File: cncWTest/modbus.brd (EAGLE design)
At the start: 39.4 x 34 mm, 12 parts, among them Q2 2N3904

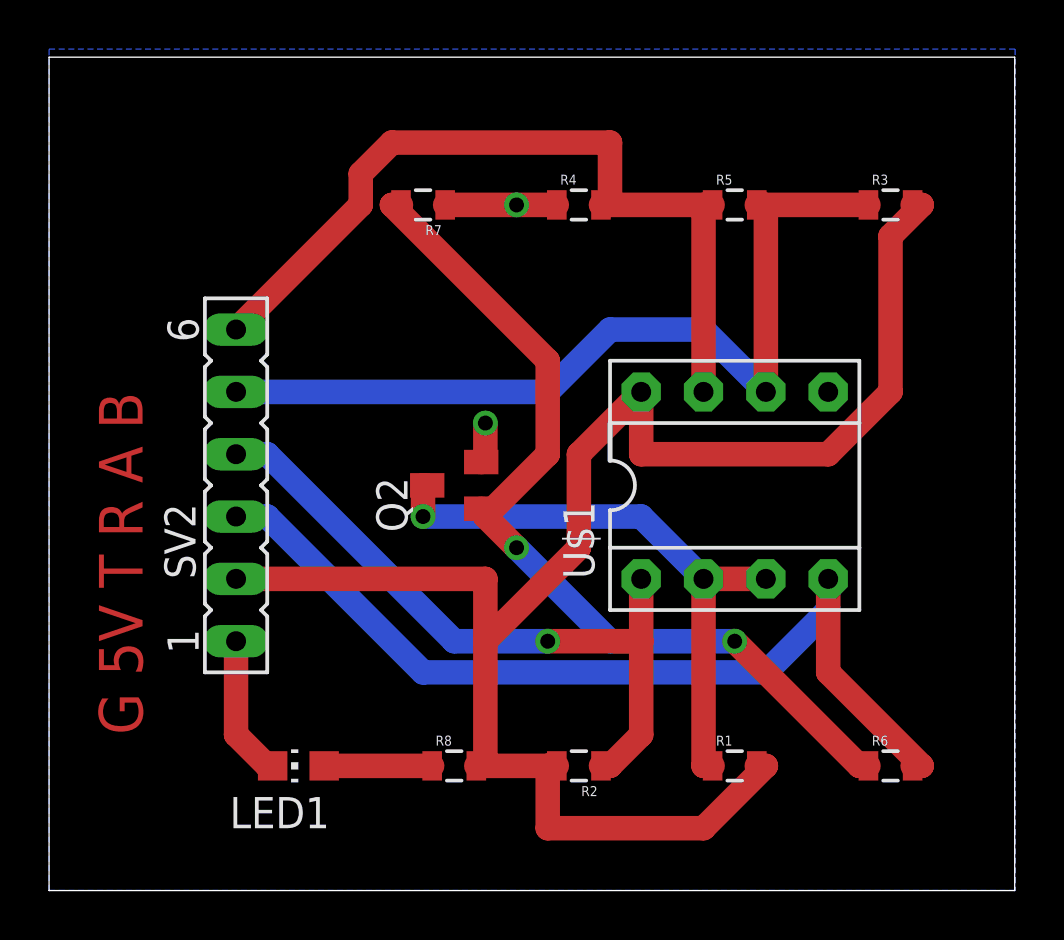
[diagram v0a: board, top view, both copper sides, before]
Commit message: CNC conf 1
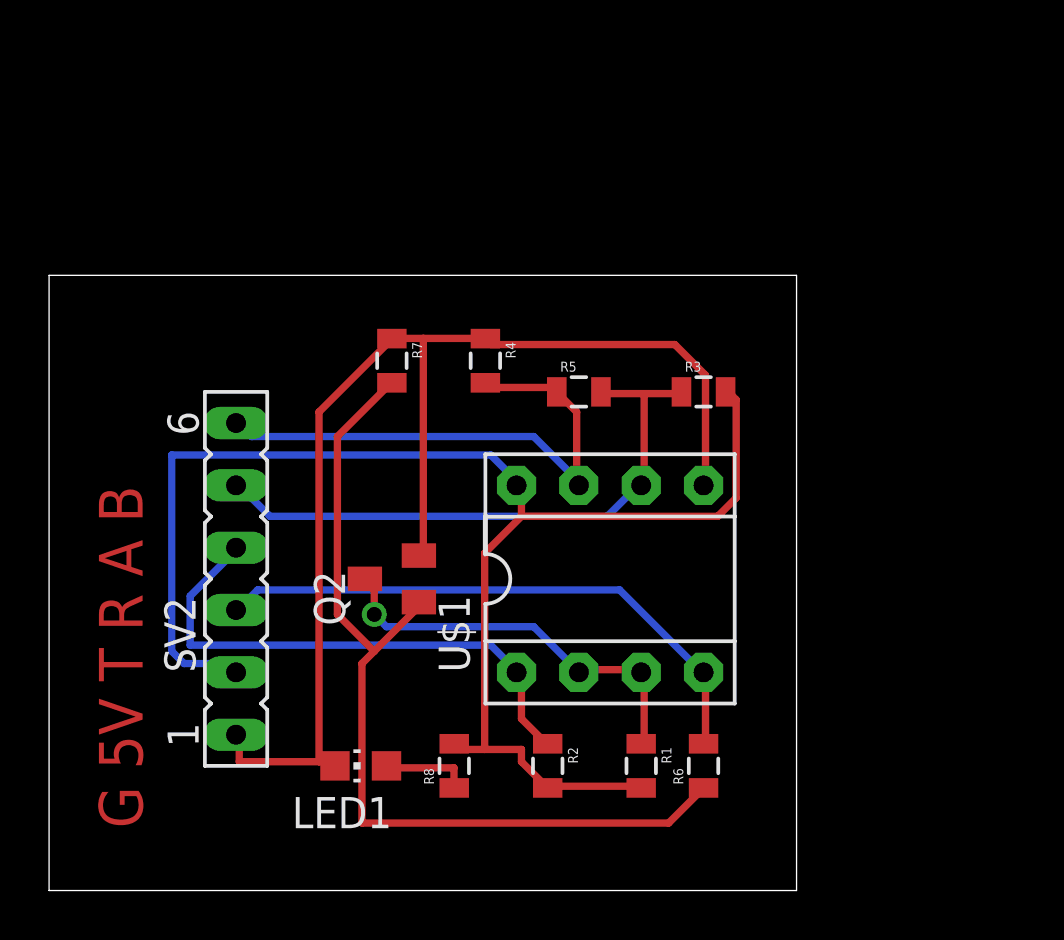
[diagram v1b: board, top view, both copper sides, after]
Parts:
- moved R3 10.8 mm to (26.7, 20.3)
- moved R5 9.92 mm to (21.6, 20.3)
- moved R6 7.62 mm to (26.7, 5.08), turned to 90 degrees
- moved R4 7.41 mm to (17.8, 21.6), turned to 270 degrees
- moved R7 6.48 mm to (14.0, 21.6), turned to 270 degrees
- moved U$1 6.35 mm to (22.9, 12.7)
- moved Q2 4.58 mm to (14.0, 12.7)
- moved R1 3.81 mm to (24.1, 5.08), turned to 270 degrees
- moved SV2 3.81 mm to (7.62, 12.7)
- moved LED1 2.54 mm to (12.7, 5.08)
- moved R2 1.27 mm to (20.3, 5.08), turned to 270 degrees
- turned R8 to 90 degrees
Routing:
- net GND: track 12.0 -> 50.5 mm, vias 2 -> 0
- net TX: track 38.7 -> 23.8 mm
- net B: track 33.9 -> 22.3 mm
- net A: track 35.9 -> 24.7 mm
- net VCC5V: track 69.0 -> 59.5 mm
- net N$2: track 24.5 -> 16.6 mm
- net RX: track 28.2 -> 22.0 mm, vias 1 -> 0
- net N$1: track 4.40 -> 3.65 mm
- net N$4: track 36.9 -> 37.0 mm, vias 2 -> 0
- removed copper zone on layer 16, net GND
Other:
- board size 39.4 x 34 mm -> 30.5 x 25.1 mm
